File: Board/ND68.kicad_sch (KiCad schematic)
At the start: 12 parts

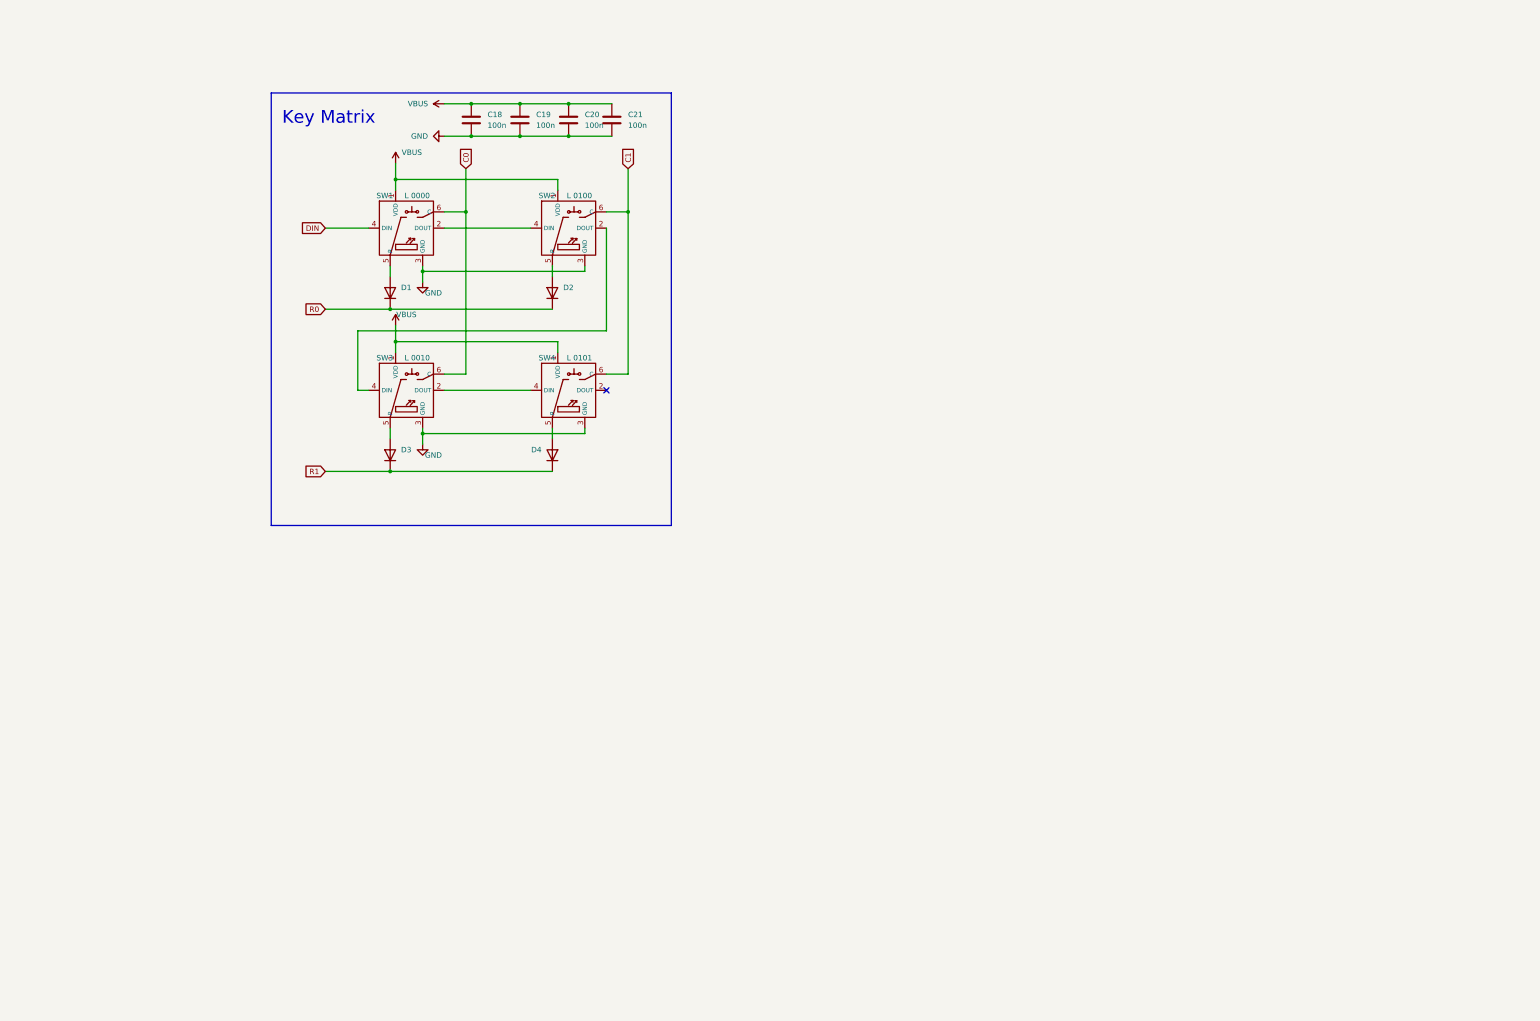
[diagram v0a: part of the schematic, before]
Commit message: 65% ke matrix
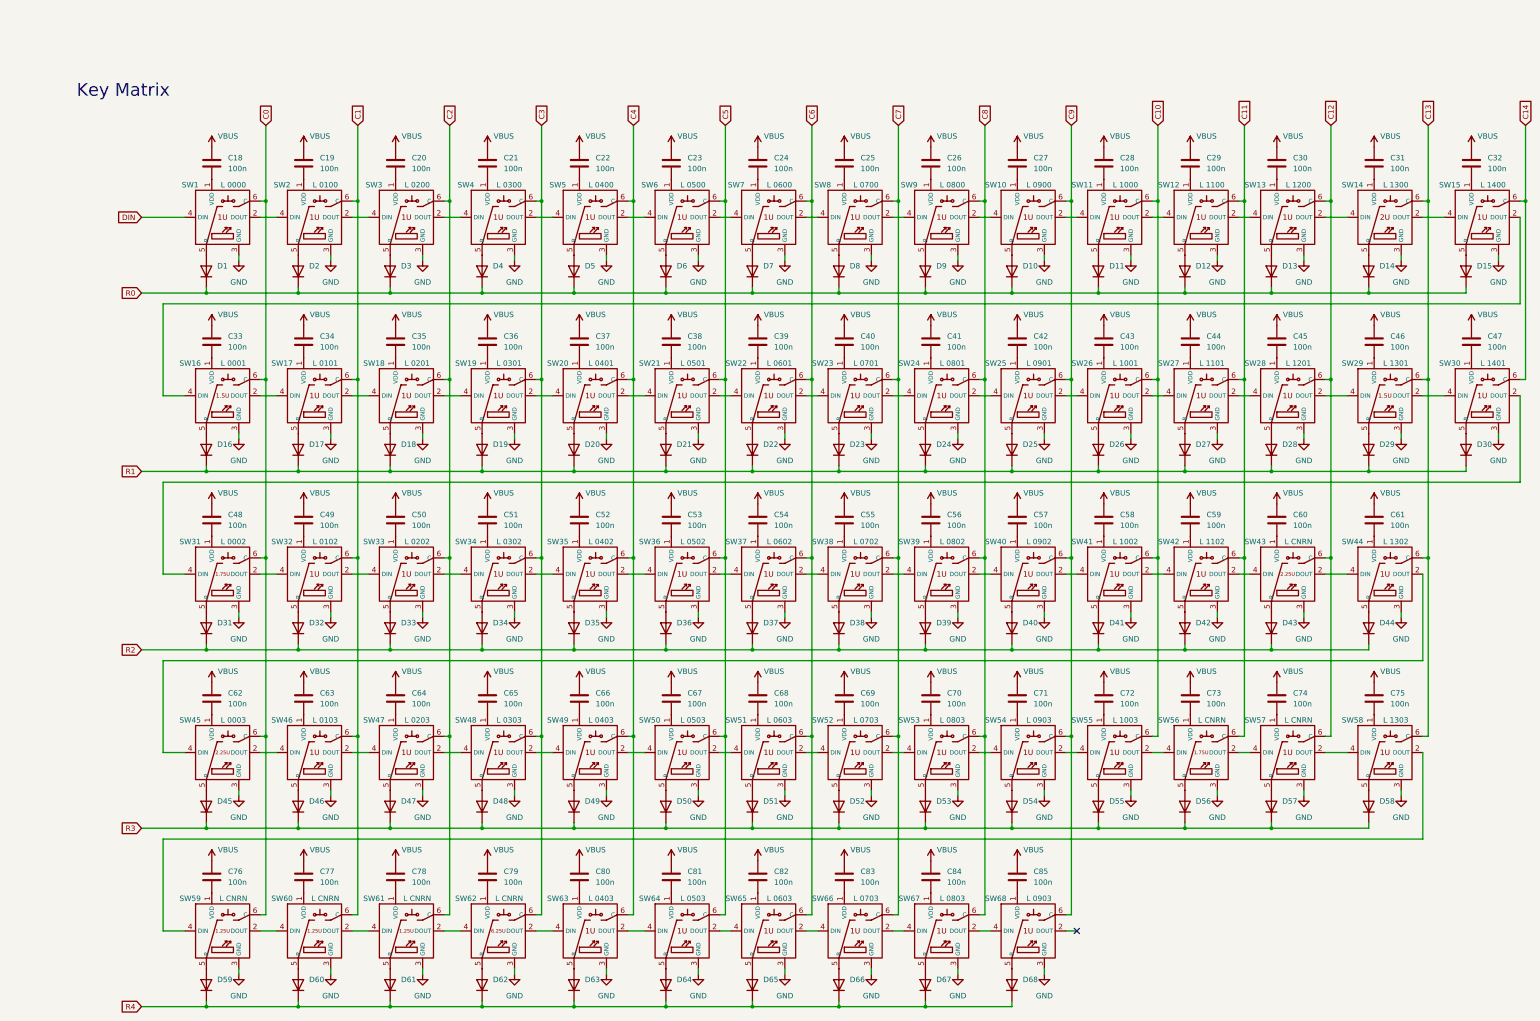
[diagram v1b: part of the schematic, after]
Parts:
- removed SW2, SW3, SW4: ~, ND68:ND68-1U-HS-ARGB, symbol ND68:nd68_hotswap_argb
- added C22, C23, C24, C25, C26, C27, C28, C29, C30, C31, C32, C33, C34, C35, C36, C37, C38, C39, C40, C41, C42, C43, C44, C45, C46, C47, C48, C49, C50, C51, C52, C53, C54, C55, C56, C57, C58, C59, C60, C61, C62, C63, C64, C65, C66, C67, C68, C69, C70, C71, C72, C73, C74, C75, C76, C77, C78, C79, C80, C81, C82, C83, C84, C85: 100n, Capacitor_SMD:C_0201_0603Metric, symbol Device:C
- added D10, D11, D12, D13, D14, D15, D16, D17, D18, D19, D20, D21, D22, D23, D24, D25, D26, D27, D28, D29, D30, D31, D32, D33, D34, D35, D36, D37, D38, D39, D40, D41, D42, D43, D44, D45, D46, D47, D48, D49, D5, D50, D51, D52, D53, D54, D55, D56, D57, D58, D59, D6, D60, D61, D62, D63, D64, D65, D66, D67, D68, D7, D8, D9: D, Diode_SMD:D_SOD-123F, symbol Device:D
- added SW10, SW11, SW12, SW13, SW15, SW17, SW18, SW19, SW2, SW20, SW21, SW22, SW23, SW24, SW25, SW26, SW27, SW28, SW3, SW30, SW32, SW33, SW34, SW35, SW36, SW37, SW38, SW39, SW4, SW40, SW41, SW42, SW44, SW46, SW47, SW48, SW49, SW5, SW50, SW51, SW52, SW53, SW54, SW55, SW57, SW58, SW6, SW63, SW64, SW65, SW66, SW67, SW68, SW7, SW8, SW9: ~, ND68:ND68-1U-HS-ARGB, symbol ND68:nd68_1u_hotswap_argb
- added SW14: ~, ND68:ND68-2U-HS-ARGB, symbol ND68:nd68_2u_hotswap_argb
- added SW16, SW29: ~, ND68:ND68-1.5U-HS-ARGB, symbol ND68:nd68_1.5u_hotswap_argb
- added SW31: ~, ND68:ND68-1.5U-HS-ARGB, symbol ND68:nd68_1.75u_hotswap_argb
- added SW43, SW45: ~, ND68:ND68-2.25U-HS-ARGB, symbol ND68:nd68_2.25u_hotswap_argb
- added SW56: ~, ND68:ND68-1.75U-HS-ARGB, symbol ND68:nd68_1.75u_hotswap_argb
- added SW59, SW60, SW61: ~, ND68:ND68-1.25U-HS-ARGB, symbol ND68:nd68_1.25u_hotswap_argb
- added SW62: ~, ND68:ND68-6.25U-HS-ARGB, symbol ND68:nd68_6.25u_hotswap_argb
- SW1: symbol ND68:nd68_hotswap_argb -> ND68:nd68_1u_hotswap_argb
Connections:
- net C0: now also SW16.6 (C), SW31.6 (C), SW45.6 (C), SW59.6 (C)
- net C1: now also SW17.6 (C), SW2.6 (C), SW32.6 (C), SW46.6 (C), SW60.6 (C)
- net GND: now also SW10.3 (GND), SW11.3 (GND), SW12.3 (GND), SW13.3 (GND), SW14.3 (GND), SW15.3 (GND), SW16.3 (GND), SW17.3 (GND), SW18.3 (GND), SW19.3 (GND), SW2.3 (GND), SW20.3 (GND), SW21.3 (GND), SW22.3 (GND), SW23.3 (GND), SW24.3 (GND), SW25.3 (GND), SW26.3 (GND), SW27.3 (GND), SW28.3 (GND), SW29.3 (GND), SW3.3 (GND), SW30.3 (GND), SW31.3 (GND), SW32.3 (GND), SW33.3 (GND), SW34.3 (GND), SW35.3 (GND), SW36.3 (GND), SW37.3 (GND), SW38.3 (GND), SW39.3 (GND), SW4.3 (GND), SW40.3 (GND), SW41.3 (GND), SW42.3 (GND), SW43.3 (GND), SW44.3 (GND), SW45.3 (GND), SW46.3 (GND), SW47.3 (GND), SW48.3 (GND), SW49.3 (GND), SW5.3 (GND), SW50.3 (GND), SW51.3 (GND), SW52.3 (GND), SW53.3 (GND), SW54.3 (GND), SW55.3 (GND), SW56.3 (GND), SW57.3 (GND), SW58.3 (GND), SW59.3 (GND), SW6.3 (GND), SW60.3 (GND), SW61.3 (GND), SW62.3 (GND), SW63.3 (GND), SW64.3 (GND), SW65.3 (GND), SW66.3 (GND), SW67.3 (GND), SW68.3 (GND), SW7.3 (GND), SW8.3 (GND), SW9.3 (GND); no longer C18.2, C19.2, C20.2, C21.2
- net R0: now also D3.1 (K), D4.1 (K), D10.1 (K), D11.1 (K), D12.1 (K), D13.1 (K), D14.1 (K), D15.1 (K), D5.1 (K), D6.1 (K), D7.1 (K), D8.1 (K), D9.1 (K)
- net R1: now also D16.1 (K), D17.1 (K), D18.1 (K), D19.1 (K), D20.1 (K), D21.1 (K), D22.1 (K), D23.1 (K), D24.1 (K), D25.1 (K), D26.1 (K), D27.1 (K), D28.1 (K), D29.1 (K), D30.1 (K); no longer D3.1 (K), D4.1 (K)
- net VBUS: now also C22.1, C23.1, C24.1, C25.1, C26.1, C27.1, C28.1, C29.1, C30.1, C31.1, C32.1, C33.1, C34.1, C35.1, C36.1, C37.1, C38.1, C39.1, C40.1, C41.1, C42.1, C43.1, C44.1, C45.1, C46.1, C47.1, C48.1, C49.1, C50.1, C51.1, C52.1, C53.1, C54.1, C55.1, C56.1, C57.1, C58.1, C59.1, C60.1, C61.1, C62.1, C63.1, C64.1, C65.1, C66.1, C67.1, C68.1, C69.1, C70.1, C71.1, C72.1, C73.1, C74.1, C75.1, C76.1, C77.1, C78.1, C79.1, C80.1, C81.1, C82.1, C83.1, C84.1, C85.1; no longer SW1.1 (VDD)
- net at D4.2 (A): now also SW4.5 (R)
- net at D2.2 (A): now also SW2.5 (R)
- net at D3.2 (A): now also SW3.5 (R)
- net at SW1.2 (DOUT): now also SW2.4 (DIN)
- new net: D48.2 (A), SW48.5 (R)
- new net: D9.2 (A), SW9.5 (R)
- new net: D66.2 (A), SW66.5 (R)
- new net: C65.2, SW48.1 (VDD)
- new net: C33.2, SW16.1 (VDD)
- new net: SW16.2 (DOUT), SW17.4 (DIN)
- new net: SW15.2 (DOUT), SW16.4 (DIN)
- new net: D16.2 (A), SW16.5 (R)
- new net: C55.2, SW38.1 (VDD)
- new net: SW38.2 (DOUT), SW39.4 (DIN)
- new net: SW37.2 (DOUT), SW38.4 (DIN)
- new net: D38.2 (A), SW38.5 (R)
- new net: C72.2, SW55.1 (VDD)
- new net: D56.2 (A), SW56.5 (R)
- new net: D29.2 (A), SW29.5 (R)
- new net: C50.2, SW33.1 (VDD)
- new net: C62.2, SW45.1 (VDD)
- new net: D46.2 (A), SW46.5 (R)
- new net: C56.2, SW39.1 (VDD)
- new net: D60.2 (A), SW60.5 (R)
- new net: D43.2 (A), SW43.5 (R)
- new net: C57.2, SW40.1 (VDD)
- new net: C32.2, SW15.1 (VDD)
- new net: SW14.2 (DOUT), SW15.4 (DIN)
- new net: D15.2 (A), SW15.5 (R)
- new net: C71.2, SW54.1 (VDD)
- new net: SW54.2 (DOUT), SW55.4 (DIN)
- new net: SW53.2 (DOUT), SW54.4 (DIN)
- new net: D54.2 (A), SW54.5 (R)
- new net: C59.2, SW42.1 (VDD)
- new net: SW42.2 (DOUT), SW43.4 (DIN)
- new net: SW41.2 (DOUT), SW42.4 (DIN)
- new net: D42.2 (A), SW42.5 (R)
- new net: D39.2 (A), SW39.5 (R)
- new net: D31.2 (A), SW31.5 (R)
- new net: C38.2, SW21.1 (VDD)
- new net: C39.2, SW22.1 (VDD)
- new net: C23.2, SW6.1 (VDD)
- new net: C52.2, SW35.1 (VDD)
- new net: C63.2, SW46.1 (VDD)
- new net: SW46.2 (DOUT), SW47.4 (DIN)
- new net: SW45.2 (DOUT), SW46.4 (DIN)
- new net: C37.2, SW20.1 (VDD)
- new net: C67.2, SW50.1 (VDD)
- new net: D30.2 (A), SW30.5 (R)
- new net: D53.2 (A), SW53.5 (R)
- new net: C78.2, SW61.1 (VDD)
- new net: SW61.2 (DOUT), SW62.4 (DIN)
- new net: SW60.2 (DOUT), SW61.4 (DIN)
- new net: D61.2 (A), SW61.5 (R)
- new net: C43.2, SW26.1 (VDD)
- new net: SW26.2 (DOUT), SW27.4 (DIN)
- new net: SW25.2 (DOUT), SW26.4 (DIN)
- new net: D26.2 (A), SW26.5 (R)
- new net: D33.2 (A), SW33.5 (R)
- new net: C31.2, SW14.1 (VDD)
- new net: D64.2 (A), SW64.5 (R)
- new net: C40.2, SW23.1 (VDD)
- new net: SW23.2 (DOUT), SW24.4 (DIN)
- new net: SW22.2 (DOUT), SW23.4 (DIN)
- new net: D23.2 (A), SW23.5 (R)
- new net: C36.2, SW19.1 (VDD)
- new net: D58.2 (A), SW58.5 (R)
- new net: C44.2, SW27.1 (VDD)
- new net: SW27.2 (DOUT), SW28.4 (DIN)
- new net: D27.2 (A), SW27.5 (R)
- new net: C79.2, SW62.1 (VDD)
- new net: SW62.2 (DOUT), SW63.4 (DIN)
- new net: D62.2 (A), SW62.5 (R)
- new net: D14.2 (A), SW14.5 (R)
- new net: C20.2, SW3.1 (VDD)
- new net: SW3.2 (DOUT), SW4.4 (DIN)
- new net: SW2.2 (DOUT), SW3.4 (DIN)
- new net: C83.2, SW66.1 (VDD)
- new net: D37.2 (A), SW37.5 (R)
- new net: C48.2, SW31.1 (VDD)
- new net: SW31.2 (DOUT), SW32.4 (DIN)
- new net: SW30.2 (DOUT), SW31.4 (DIN)
- new net: D19.2 (A), SW19.5 (R)
- new net: C61.2, SW44.1 (VDD)
- new net: SW44.2 (DOUT), SW45.4 (DIN)
- new net: SW43.2 (DOUT), SW44.4 (DIN)
- new net: D44.2 (A), SW44.5 (R)
- new net: C47.2, SW30.1 (VDD)
- new net: C70.2, SW53.1 (VDD)
- new net: SW52.2 (DOUT), SW53.4 (DIN)
- new net: C53.2, SW36.1 (VDD)
- new net: C81.2, SW64.1 (VDD)
- new net: SW64.2 (DOUT), SW65.4 (DIN)
- new net: SW63.2 (DOUT), SW64.4 (DIN)
- new net: C68.2, SW51.1 (VDD)
- new net: D65.2 (A), SW65.5 (R)
- new net: C58.2, SW41.1 (VDD)
- new net: SW40.2 (DOUT), SW41.4 (DIN)
- new net: D41.2 (A), SW41.5 (R)
- new net: SW33.2 (DOUT), SW34.4 (DIN)
- new net: SW32.2 (DOUT), SW33.4 (DIN)
- new net: C60.2, SW43.1 (VDD)
- new net: C25.2, SW8.1 (VDD)
- new net: C49.2, SW32.1 (VDD)
- new net: SW50.2 (DOUT), SW51.4 (DIN)
- new net: SW49.2 (DOUT), SW50.4 (DIN)
- new net: D50.2 (A), SW50.5 (R)
- new net: C69.2, SW52.1 (VDD)
- new net: SW51.2 (DOUT), SW52.4 (DIN)
- new net: D52.2 (A), SW52.5 (R)
- new net: C76.2, SW59.1 (VDD)
- new net: SW59.2 (DOUT), SW60.4 (DIN)
- new net: SW58.2 (DOUT), SW59.4 (DIN)
- new net: D59.2 (A), SW59.5 (R)
- new net: SW13.2 (DOUT), SW14.4 (DIN)
- new net: C66.2, SW49.1 (VDD)
- new net: SW48.2 (DOUT), SW49.4 (DIN)
- new net: D49.2 (A), SW49.5 (R)
- new net: D47.2 (A), SW47.5 (R)
- new net: D36.2 (A), SW36.5 (R)
- new net: C77.2, SW60.1 (VDD)
- new net: D6.2 (A), SW6.5 (R)
- new net: D55.2 (A), SW55.5 (R)
- new net: SW39.2 (DOUT), SW40.4 (DIN)
- new net: C34.2, SW17.1 (VDD)
- new net: SW17.2 (DOUT), SW18.4 (DIN)
- new net: D17.2 (A), SW17.5 (R)
- new net: D34.2 (A), SW34.5 (R)
- new net: D40.2 (A), SW40.5 (R)
- new net: C27.2, SW10.1 (VDD)
- new net: SW10.2 (DOUT), SW11.4 (DIN)
- new net: SW10.4 (DIN), SW9.2 (DOUT)
- new net: D10.2 (A), SW10.5 (R)
- new net: D51.2 (A), SW51.5 (R)
- new net: SW21.2 (DOUT), SW22.4 (DIN)
- new net: SW20.2 (DOUT), SW21.4 (DIN)
- new net: D21.2 (A), SW21.5 (R)
- new net: D24.2 (A), SW24.5 (R)
- new net: C42.2, SW25.1 (VDD)
- new net: SW24.2 (DOUT), SW25.4 (DIN)
- new net: D25.2 (A), SW25.5 (R)
- new net: SW6.2 (DOUT), SW7.4 (DIN)
- new net: SW5.2 (DOUT), SW6.4 (DIN)
- new net: C54.2, SW37.1 (VDD)
- new net: SW36.2 (DOUT), SW37.4 (DIN)
- new net: C74.2, SW57.1 (VDD)
- new net: SW57.2 (DOUT), SW58.4 (DIN)
- new net: SW56.2 (DOUT), SW57.4 (DIN)
- new net: D57.2 (A), SW57.5 (R)
- new net: D28.2 (A), SW28.5 (R)
- new net: C64.2, SW47.1 (VDD)
- new net: D63.2 (A), SW63.5 (R)
- new net: C21.2, SW4.1 (VDD)
- new net: SW4.2 (DOUT), SW5.4 (DIN)
- new net: SW29.2 (DOUT), SW30.4 (DIN)
- new net: C22.2, SW5.1 (VDD)
- new net: D68.2 (A), SW68.5 (R)
- new net: C45.2, SW28.1 (VDD)
- new net: SW28.2 (DOUT), SW29.4 (DIN)
- new net: C28.2, SW11.1 (VDD)
- new net: SW11.2 (DOUT), SW12.4 (DIN)
- new net: D11.2 (A), SW11.5 (R)
- new net: D5.2 (A), SW5.5 (R)
- new net: C24.2, SW7.1 (VDD)
- new net: SW7.2 (DOUT), SW8.4 (DIN)
- new net: D7.2 (A), SW7.5 (R)
- new net: C41.2, SW24.1 (VDD)
- new net: D12.2 (A), SW12.5 (R)
- new net: C19.2, SW2.1 (VDD)
- new net: C29.2, SW12.1 (VDD)
- new net: SW12.2 (DOUT), SW13.4 (DIN)
- new net: C80.2, SW63.1 (VDD)
- new net: C51.2, SW34.1 (VDD)
- new net: SW34.2 (DOUT), SW35.4 (DIN)
- new net: D32.2 (A), SW32.5 (R)
- new net: D67.2 (A), SW67.5 (R)
- new net: C85.2, SW68.1 (VDD)
- new net: SW67.2 (DOUT), SW68.4 (DIN)
- new net: D8.2 (A), SW8.5 (R)
- new net: C75.2, SW58.1 (VDD)
- new net: C18.2, SW1.1 (VDD)
- new net: D13.2 (A), SW13.5 (R)
- new net: D22.2 (A), SW22.5 (R)
- new net: C84.2, SW67.1 (VDD)
- new net: C30.2, SW13.1 (VDD)
- new net: C46.2, SW29.1 (VDD)
- new net: C73.2, SW56.1 (VDD)
- new net: SW19.2 (DOUT), SW20.4 (DIN)
- new net: SW18.2 (DOUT), SW19.4 (DIN)
- new net: SW47.2 (DOUT), SW48.4 (DIN)
- new net: SW55.2 (DOUT), SW56.4 (DIN)
- new net: SW66.2 (DOUT), SW67.4 (DIN)
- new net: SW65.2 (DOUT), SW66.4 (DIN)
- new net: SW35.2 (DOUT), SW36.4 (DIN)
- new net: C82.2, SW65.1 (VDD)
- new net: C26.2, SW9.1 (VDD)
- new net: SW8.2 (DOUT), SW9.4 (DIN)
- new net: D20.2 (A), SW20.5 (R)
- new net: C35.2, SW18.1 (VDD)
- new net: D18.2 (A), SW18.5 (R)
- new net: D45.2 (A), SW45.5 (R)
- new net: D35.2 (A), SW35.5 (R)
- new net C10: SW11.6 (C), SW26.6 (C), SW41.6 (C), SW55.6 (C)
- new net C11: SW12.6 (C), SW27.6 (C), SW42.6 (C), SW56.6 (C)
- new net C12: SW13.6 (C), SW28.6 (C), SW43.6 (C), SW57.6 (C)
- new net C13: SW14.6 (C), SW29.6 (C), SW44.6 (C), SW58.6 (C)
- new net C14: SW15.6 (C), SW30.6 (C)
- new net C2: SW18.6 (C), SW3.6 (C), SW33.6 (C), SW47.6 (C), SW61.6 (C)
- new net C3: SW19.6 (C), SW34.6 (C), SW4.6 (C), SW48.6 (C), SW62.6 (C)
- new net C4: SW20.6 (C), SW35.6 (C), SW49.6 (C), SW5.6 (C), SW63.6 (C)
- new net C5: SW21.6 (C), SW36.6 (C), SW50.6 (C), SW6.6 (C), SW64.6 (C)
- new net C6: SW22.6 (C), SW37.6 (C), SW51.6 (C), SW65.6 (C), SW7.6 (C)
- new net C7: SW23.6 (C), SW38.6 (C), SW52.6 (C), SW66.6 (C), SW8.6 (C)
- new net C8: SW24.6 (C), SW39.6 (C), SW53.6 (C), SW67.6 (C), SW9.6 (C)
- new net C9: SW10.6 (C), SW25.6 (C), SW40.6 (C), SW54.6 (C), SW68.6 (C)
- new net R2: D31.1 (K), D32.1 (K), D33.1 (K), D34.1 (K), D35.1 (K), D36.1 (K), D37.1 (K), D38.1 (K), D39.1 (K), D40.1 (K), D41.1 (K), D42.1 (K), D43.1 (K), D44.1 (K)
- new net R3: D45.1 (K), D46.1 (K), D47.1 (K), D48.1 (K), D49.1 (K), D50.1 (K), D51.1 (K), D52.1 (K), D53.1 (K), D54.1 (K), D55.1 (K), D56.1 (K), D57.1 (K), D58.1 (K)
- new net R4: D59.1 (K), D60.1 (K), D61.1 (K), D62.1 (K), D63.1 (K), D64.1 (K), D65.1 (K), D66.1 (K), D67.1 (K), D68.1 (K)
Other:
- moved on the sheet: C18, D1
